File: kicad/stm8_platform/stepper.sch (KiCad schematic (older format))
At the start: 32 parts, among them J1 CONN_02X10, P1 UART, P2 SWIM, Q1 AO3401, Q2 AO3401, Q3 AO3401, SW1 SW_DIP_x03, U1 STM8S105K4T6C, U2 ULN2803A, U3 LD1117S50CTR

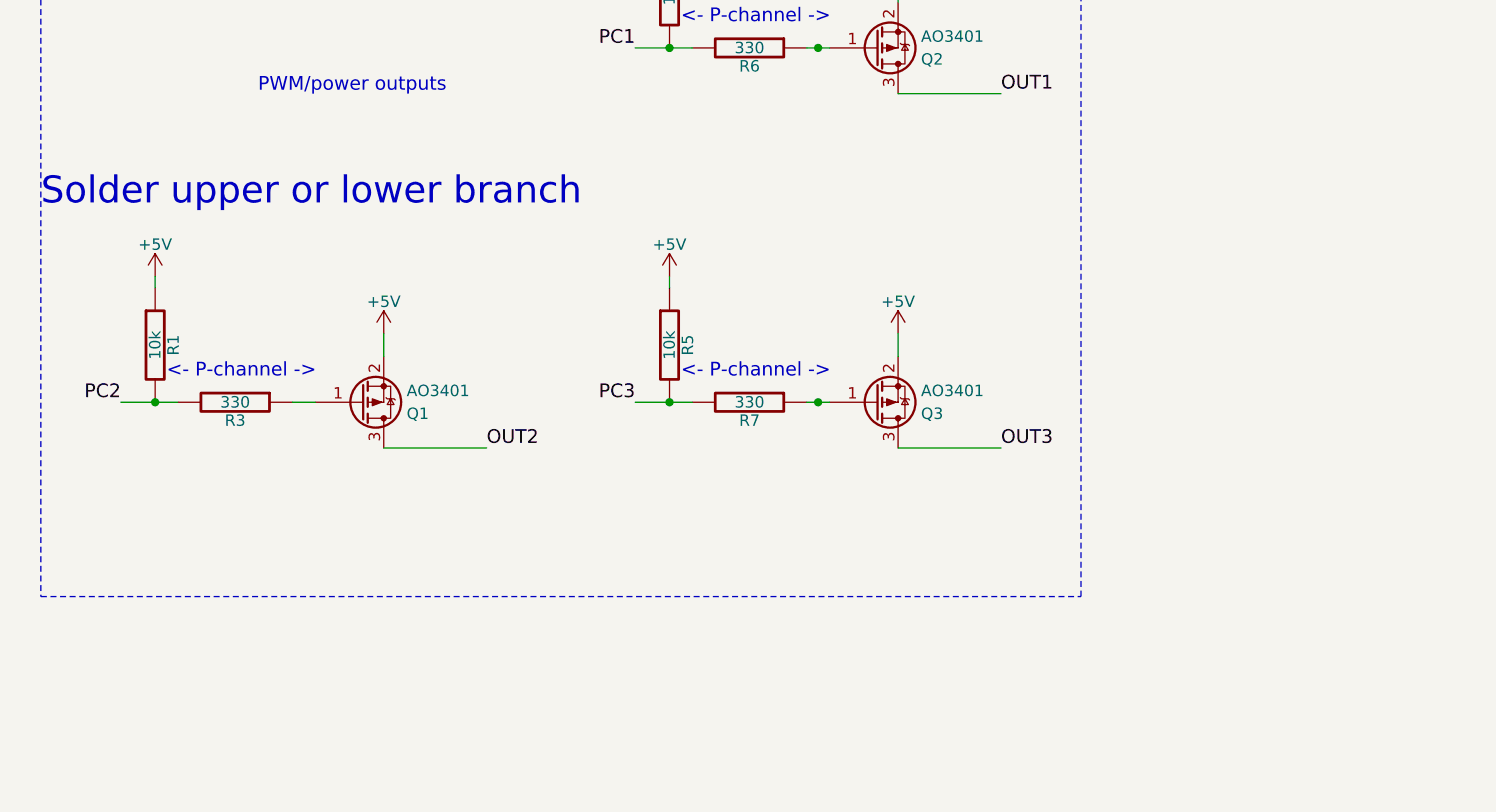
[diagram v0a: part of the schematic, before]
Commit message: small update
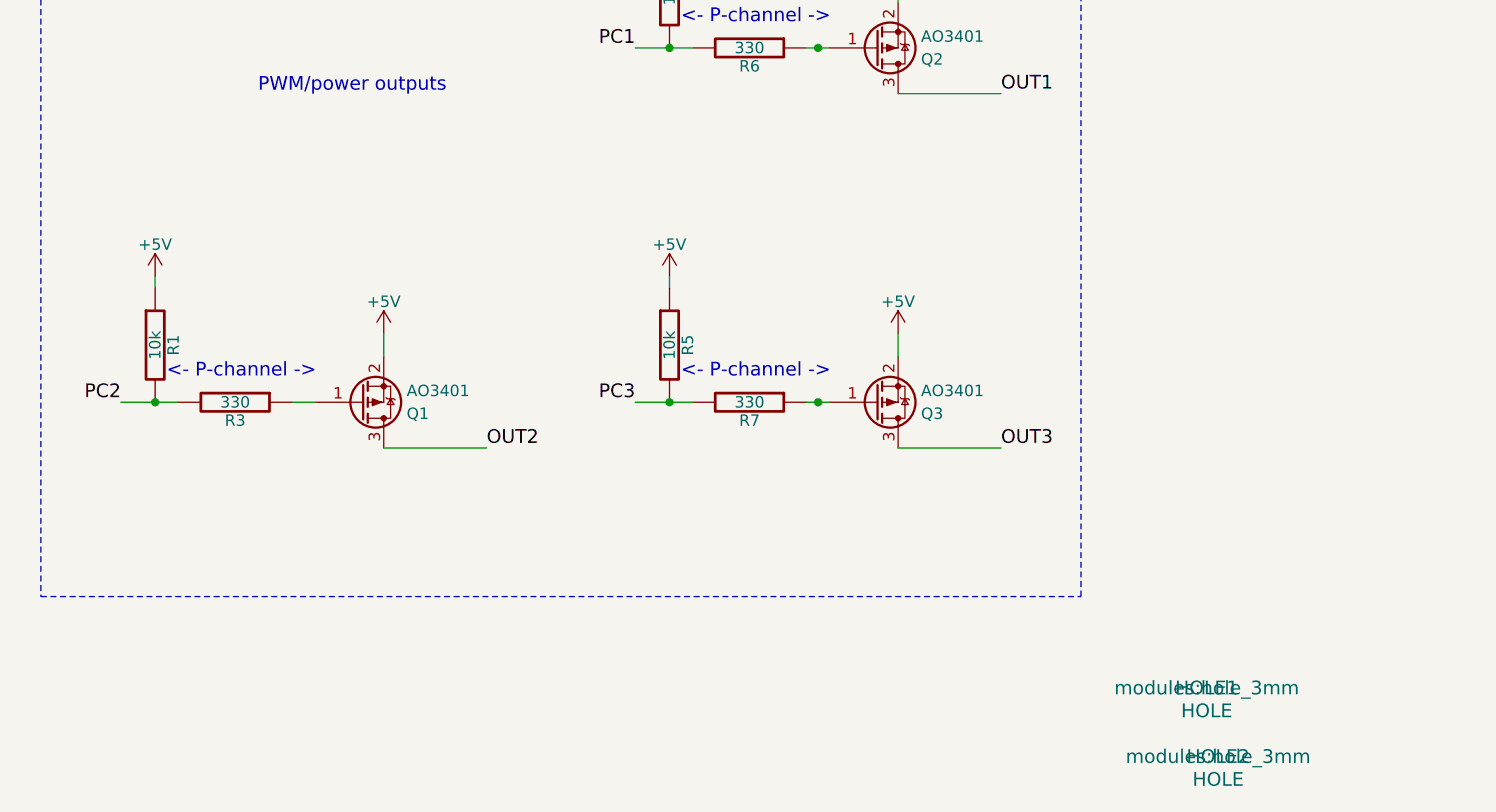
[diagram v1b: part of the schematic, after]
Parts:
- added HOLE1, HOLE2: HOLE, modules:hole_3mm, symbol HOLE
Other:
- note removed: "Solder upper or lower branch"
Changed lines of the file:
@@
 LIBS:switches
 LIBS:ESD_Protection
+LIBS:my_elements
 LIBS:stepper-cache
 EELAYER 25 0
@@
 $EndComp
 $Comp
-L GND-RESCUE-stepper #PWR01
+L GND-RESCUE-stepper #PWR5
 U 1 1 52FB03EF
 P 1500 1950
-F 0 "#PWR01" H 1500 1950 30  0001 C CNN
+F 0 "#PWR5" H 1500 1950 30  0001 C CNN
 F 1 "GND" H 1500 1880 30  0001 C CNN
 F 2 "" H 1500 1950 60  0000 C CNN
@@
 $EndComp
 $Comp
-L GND-RESCUE-stepper #PWR02
+L GND-RESCUE-stepper #PWR4
 U 1 1 52FB0400
 P 1500 1350
-F 0 "#PWR02" H 1500 1350 30  0001 C CNN
+F 0 "#PWR4" H 1500 1350 30  0001 C CNN
 F 1 "GND" H 1500 1280 30  0001 C CNN
 F 2 "" H 1500 1350 60  0000 C CNN
@@
 $EndComp
 $Comp
-L GND-RESCUE-stepper #PWR03
+L GND-RESCUE-stepper #PWR1
 U 1 1 52FB0453
 P 800 1850
-F 0 "#PWR03" H 800 1850 30  0001 C CNN
+F 0 "#PWR1" H 800 1850 30  0001 C CNN
 F 1 "GND" H 800 1780 30  0001 C CNN
 F 2 "" H 800 1850 60  0000 C CNN
@@
 $EndComp
 $Comp
-L GND-RESCUE-stepper #PWR04
+L GND-RESCUE-stepper #PWR22
 U 1 1 52FB0F03
 P 9850 1650
-F 0 "#PWR04" H 9850 1650 30  0001 C CNN
+F 0 "#PWR22" H 9850 1650 30  0001 C CNN
 F 1 "GND" H 9850 1580 30  0001 C CNN
 F 2 "" H 9850 1650 60  0000 C CNN
@@
 $EndComp
 $Comp
-L GND-RESCUE-stepper #PWR05
+L GND-RESCUE-stepper #PWR23
 U 1 1 52FB287C
 P 10150 1400
-F 0 "#PWR05" H 10150 1400 30  0001 C CNN
+F 0 "#PWR23" H 10150 1400 30  0001 C CNN
 F 1 "GND" H 10150 1330 30  0001 C CNN
 F 2 "" H 10150 1400 60  0000 C CNN
@@
 TXD
 $Comp
-L GND-RESCUE-stepper #PWR06
+L GND-RESCUE-stepper #PWR26
 U 1 1 52FB4CEF
 P 10650 2500
-F 0 "#PWR06" H 10650 2500 30  0001 C CNN
+F 0 "#PWR26" H 10650 2500 30  0001 C CNN
 F 1 "GND" H 10650 2430 30  0001 C CNN
 F 2 "" H 10650 2500 60  0000 C CNN
@@
 $EndComp
 $Comp
-L +5V #PWR07
+L +5V #PWR20
 U 1 1 5984240F
 P 9250 1050
-F 0 "#PWR07" H 9250 900 50  0001 C CNN
+F 0 "#PWR20" H 9250 900 50  0001 C CNN
 F 1 "+5V" H 9250 1190 50  0000 C CNN
 F 2 "" H 9250 1050 50  0001 C CNN
@@
 $EndComp
 $Comp
-L +5V #PWR08
+L +5V #PWR25
 U 1 1 59842472
 P 10600 1600
-F 0 "#PWR08" H 10600 1450 50  0001 C CNN
+F 0 "#PWR25" H 10600 1450 50  0001 C CNN
 F 1 "+5V" H 10600 1740 50  0000 C CNN
 F 2 "" H 10600 1600 50  0001 C CNN
@@
 $EndComp
 $Comp
-L +5V #PWR09
+L +5V #PWR2
 U 1 1 598424AD
 P 1350 1750
-F 0 "#PWR09" H 1350 1600 50  0001 C CNN
+F 0 "#PWR2" H 1350 1600 50  0001 C CNN
 F 1 "+5V" H 1350 1890 50  0000 C CNN
 F 2 "" H 1350 1750 50  0001 C CNN
@@
 $EndComp
 $Comp
-L +5V #PWR010
+L +5V #PWR7
 U 1 1 59842925
 P 2500 3650
-F 0 "#PWR010" H 2500 3500 50  0001 C CNN
+F 0 "#PWR7" H 2500 3500 50  0001 C CNN
 F 1 "+5V" H 2500 3790 50  0000 C CNN
 F 2 "" H 2500 3650 50  0001 C CNN
@@
 $EndComp
 $Comp
-L +5V #PWR011
+L +5V #PWR21
 U 1 1 59844ACD
 P 9400 3650
-F 0 "#PWR011" H 9400 3500 50  0001 C CNN
+F 0 "#PWR21" H 9400 3500 50  0001 C CNN
 F 1 "+5V" H 9400 3790 50  0000 C CNN
 F 2 "" H 9400 3650 50  0001 C CNN
@@
 $EndComp
 $Comp
-L GND-RESCUE-stepper #PWR012
+L GND-RESCUE-stepper #PWR27
 U 1 1 598456D9
 P 10700 3200
-F 0 "#PWR012" H 10700 3200 30  0001 C CNN
+F 0 "#PWR27" H 10700 3200 30  0001 C CNN
 F 1 "GND" H 10700 3130 30  0001 C CNN
 F 2 "" H 10700 3200 60  0000 C CNN
@@
 On-board LED
 $Comp
-L +5V #PWR013
+L +5V #PWR3
 U 1 1 59847EEF
 P 1350 5100
-F 0 "#PWR013" H 1350 4950 50  0001 C CNN
+F 0 "#PWR3" H 1350 4950 50  0001 C CNN
 F 1 "+5V" H 1350 5240 50  0000 C CNN
 F 2 "" H 1350 5100 50  0001 C CNN
@@
 $EndComp
 $Comp
-L +5V #PWR014
+L +5V #PWR6
 U 1 1 59848624
 P 2350 5350
-F 0 "#PWR014" H 2350 5200 50  0001 C CNN
+F 0 "#PWR6" H 2350 5200 50  0001 C CNN
 F 1 "+5V" H 2350 5490 50  0000 C CNN
 F 2 "" H 2350 5350 50  0001 C CNN
@@
 5.0V
 $Comp
-L +5V #PWR015
+L +5V #PWR24
 U 1 1 598515D1
 P 10250 2700
-F 0 "#PWR015" H 10250 2550 50  0001 C CNN
+F 0 "#PWR24" H 10250 2550 50  0001 C CNN
 F 1 "+5V" H 10250 2840 50  0000 C CNN
 F 2 "" H 10250 2700 50  0001 C CNN
@@
 $EndComp
 $Comp
-L GND-RESCUE-stepper #PWR016
+L GND-RESCUE-stepper #PWR16
 U 1 1 598534FD
 P 8200 1600
-F 0 "#PWR016" H 8200 1600 30  0001 C CNN
+F 0 "#PWR16" H 8200 1600 30  0001 C CNN
 F 1 "GND" H 8200 1530 30  0001 C CNN
 F 2 "" H 8200 1600 60  0000 C CNN
@@
 $EndComp
 $Comp
-L +5V #PWR017
+L +5V #PWR18
 U 1 1 59853D62
 P 8800 1100
-F 0 "#PWR017" H 8800 950 50  0001 C CNN
+F 0 "#PWR18" H 8800 950 50  0001 C CNN
 F 1 "+5V" H 8800 1240 50  0000 C CNN
 F 2 "" H 8800 1100 50  0001 C CNN
@@
 $EndComp
 $Comp
-L +12V #PWR018
+L +12V #PWR14
 U 1 1 59854294
 P 7650 1100
-F 0 "#PWR018" H 7650 950 50  0001 C CNN
+F 0 "#PWR14" H 7650 950 50  0001 C CNN
 F 1 "+12V" H 7650 1240 50  0000 C CNN
 F 2 "" H 7650 1100 50  0001 C CNN
@@
 ext USART
 $Comp
-L GND-RESCUE-stepper #PWR019
+L GND-RESCUE-stepper #PWR19
 U 1 1 598572C2
 P 9000 2650
-F 0 "#PWR019" H 9000 2650 30  0001 C CNN
+F 0 "#PWR19" H 9000 2650 30  0001 C CNN
 F 1 "GND" H 9000 2580 30  0001 C CNN
 F 2 "" H 9000 2650 60  0000 C CNN
@@
 $EndComp
 $Comp
-L GND-RESCUE-stepper #PWR020
+L GND-RESCUE-stepper #PWR12
 U 1 1 59857BB1
 P 6550 2200
-F 0 "#PWR020" H 6550 2200 30  0001 C CNN
+F 0 "#PWR12" H 6550 2200 30  0001 C CNN
 F 1 "GND" H 6550 2130 30  0001 C CNN
 F 2 "" H 6550 2200 60  0000 C CNN
@@
 $EndComp
 $Comp
-L +12V #PWR021
+L +12V #PWR13
 U 1 1 59858729
 P 7050 2050
-F 0 "#PWR021" H 7050 1900 50  0001 C CNN
+F 0 "#PWR13" H 7050 1900 50  0001 C CNN
 F 1 "+12V" H 7050 2190 50  0000 C CNN
 F 2 "" H 7050 2050 50  0001 C CNN
@@
 M2E2
 $Comp
-L +12V #PWR022
+L +12V #PWR17
 U 1 1 59864EE6
 P 8200 5500
-F 0 "#PWR022" H 8200 5350 50  0001 C CNN
+F 0 "#PWR17" H 8200 5350 50  0001 C CNN
 F 1 "+12V" H 8200 5640 50  0000 C CNN
 F 2 "" H 8200 5500 50  0001 C CNN
@@
 $EndComp
 $Comp
-L PWR_FLAG #FLG023
+L PWR_FLAG #FLG1
 U 1 1 598652F0
 P 8100 5500
-F 0 "#FLG023" H 8100 5575 50  0001 C CNN
+F 0 "#FLG1" H 8100 5575 50  0001 C CNN
 F 1 "PWR_FLAG" H 8100 5650 50  0001 C CNN
 F 2 "" H 8100 5500 50  0001 C CNN
@@
 $EndComp
 $Comp
-L GND-RESCUE-stepper #PWR024
+L GND-RESCUE-stepper #PWR15
 U 1 1 598655A5
 P 8050 4650
-F 0 "#PWR024" H 8050 4650 30  0001 C CNN
+F 0 "#PWR15" H 8050 4650 30  0001 C CNN
 F 1 "GND" H 8050 4580 30  0001 C CNN
 F 2 "" H 8050 4650 60  0000 C CNN
@@
 $EndComp
 $Comp
-L PWR_FLAG #FLG025
+L PWR_FLAG #FLG2
 U 1 1 5986564B
 P 8200 4600
-F 0 "#FLG025" H 8200 4675 50  0001 C CNN
+F 0 "#FLG2" H 8200 4675 50  0001 C CNN
 F 1 "PWR_FLAG" H 8200 4750 50  0001 C CNN
 F 2 "" H 8200 4600 50  0001 C CNN
@@
 $EndComp
 $Comp
-L +5V #PWR026
+L +5V #PWR9
 U 1 1 59875BF0
 P 3600 5100
-F 0 "#PWR026" H 3600 4950 50  0001 C CNN
+F 0 "#PWR9" H 3600 4950 50  0001 C CNN
 F 1 "+5V" H 3600 5240 50  0000 C CNN
 F 2 "" H 3600 5100 50  0001 C CNN
@@
 $EndComp
 $Comp
-L +5V #PWR027
+L +5V #PWR11
 U 1 1 59875BF6
 P 4600 5350
-F 0 "#PWR027" H 4600 5200 50  0001 C CNN
+F 0 "#PWR11" H 4600 5200 50  0001 C CNN
 F 1 "+5V" H 4600 5490 50  0000 C CNN
 F 2 "" H 4600 5350 50  0001 C CNN
@@
 $EndComp
 $Comp
-L +5V #PWR028
+L +5V #PWR8
 U 1 1 59876770
 P 3600 3550
-F 0 "#PWR028" H 3600 3400 50  0001 C CNN
+F 0 "#PWR8" H 3600 3400 50  0001 C CNN
 F 1 "+5V" H 3600 3690 50  0000 C CNN
 F 2 "" H 3600 3550 50  0001 C CNN
@@
 $EndComp
 $Comp
-L +5V #PWR029
+L +5V #PWR10
 U 1 1 59876776
 P 4600 3800
-F 0 "#PWR029" H 4600 3650 50  0001 C CNN
+F 0 "#PWR10" H 4600 3650 50  0001 C CNN
 F 1 "+5V" H 4600 3940 50  0000 C CNN
 F 2 "" H 4600 3800 50  0001 C CNN
@@
 Wire Notes Line
 	5400 3300 850  3300
-Text Notes 850  4800 0    118  ~ 0
-Solder upper or lower branch
 Wire Wire Line
 	8150 2850 8500 2850
@@
 	8600 2500 8250 2500
 Connection ~ 8250 2500
+$Comp
+L HOLE HOLE2
+U 1 1 59B6BC5E
+P 6000 7200
+F 0 "HOLE2" H 6000 7200 60  0000 C CNN
+F 1 "HOLE" H 6000 7100 60  0000 C CNN
+F 2 "modules:hole_3mm" H 6000 7200 60  0000 C CNN
+F 3 "" H 6000 7200 60  0000 C CNN
+	1    6000 7200
+	1    0    0    -1
+$EndComp
+$Comp
+L HOLE HOLE1
+U 1 1 59B6D60D
+P 5950 6900
+F 0 "HOLE1" H 5950 6900 60  0000 C CNN
+F 1 "HOLE" H 5950 6800 60  0000 C CNN
+F 2 "modules:hole_3mm" H 5950 6900 60  0000 C CNN
+F 3 "" H 5950 6900 60  0000 C CNN
+	1    5950 6900
+	1    0    0    -1
+$EndComp
 $EndSCHEMATC

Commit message: add code for STM8-based 2stepper management board
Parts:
- removed P2: SWIM, Pin_Headers.pretty:Pin_Header_Angled_1x04_Pitch2.54mm, symbol CONN_01X05
- added P2: SWIM, Connector_PinHeader_2.54mm.pretty:PinHeader_1x03_P2.54mm_Horizontal, symbol Conn_01x03
- SW1: symbol SW_DIP_x03 -> SW_DIP_x03-RESCUE-stepper
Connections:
- net GND: now also P2.3 (Pin_3)
- net NRST: now also P2.1 (Pin_1)
- net SWIM/PD1: now also P2.2 (Pin_2)
- no-connect marks 6 -> 5
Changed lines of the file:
@@
 $EndComp
 $Comp
-L GND-RESCUE-stepper #PWR5
+L GND-RESCUE-stepper #PWR01
 U 1 1 52FB03EF
 P 1500 1950
-F 0 "#PWR5" H 1500 1950 30  0001 C CNN
+F 0 "#PWR01" H 1500 1950 30  0001 C CNN
 F 1 "GND" H 1500 1880 30  0001 C CNN
 F 2 "" H 1500 1950 60  0000 C CNN
@@
 $EndComp
 $Comp
-L GND-RESCUE-stepper #PWR4
+L GND-RESCUE-stepper #PWR02
 U 1 1 52FB0400
 P 1500 1350
-F 0 "#PWR4" H 1500 1350 30  0001 C CNN
+F 0 "#PWR02" H 1500 1350 30  0001 C CNN
 F 1 "GND" H 1500 1280 30  0001 C CNN
 F 2 "" H 1500 1350 60  0000 C CNN
@@
 $EndComp
 $Comp
-L GND-RESCUE-stepper #PWR1
+L GND-RESCUE-stepper #PWR03
 U 1 1 52FB0453
 P 800 1850
-F 0 "#PWR1" H 800 1850 30  0001 C CNN
+F 0 "#PWR03" H 800 1850 30  0001 C CNN
 F 1 "GND" H 800 1780 30  0001 C CNN
 F 2 "" H 800 1850 60  0000 C CNN
@@
 Text Label 4550 1000 0    60   ~ 0
 PD7
-$Comp
-L CONN_01X05 P2
-U 1 1 52FB0A49
-P 10900 1350
-F 0 "P2" H 10900 1650 50  0000 C CNN
-F 1 "SWIM" H 10900 1050 50  0000 C CNN
-F 2 "Pin_Headers.pretty:Pin_Header_Angled_1x04_Pitch2.54mm" H 10900 1350 60  0001 C CNN
-F 3 "" H 10900 1350 60  0000 C CNN
-	1    10900 1350
-	1    0    0    -1
-$EndComp
 Text Label 10700 1250 2    60   ~ 0
 SWIM/PD1
@@
 $EndComp
 $Comp
-L GND-RESCUE-stepper #PWR22
+L GND-RESCUE-stepper #PWR04
 U 1 1 52FB0F03
 P 9850 1650
-F 0 "#PWR22" H 9850 1650 30  0001 C CNN
+F 0 "#PWR04" H 9850 1650 30  0001 C CNN
 F 1 "GND" H 9850 1580 30  0001 C CNN
 F 2 "" H 9850 1650 60  0000 C CNN
@@
 $EndComp
 $Comp
-L GND-RESCUE-stepper #PWR23
+L GND-RESCUE-stepper #PWR05
 U 1 1 52FB287C
 P 10150 1400
-F 0 "#PWR23" H 10150 1400 30  0001 C CNN
+F 0 "#PWR05" H 10150 1400 30  0001 C CNN
 F 1 "GND" H 10150 1330 30  0001 C CNN
 F 2 "" H 10150 1400 60  0000 C CNN
@@
 TXD
 $Comp
-L GND-RESCUE-stepper #PWR26
+L GND-RESCUE-stepper #PWR06
 U 1 1 52FB4CEF
 P 10650 2500
-F 0 "#PWR26" H 10650 2500 30  0001 C CNN
+F 0 "#PWR06" H 10650 2500 30  0001 C CNN
 F 1 "GND" H 10650 2430 30  0001 C CNN
 F 2 "" H 10650 2500 60  0000 C CNN
@@
 $EndComp
 $Comp
-L SW_DIP_x03 SW1
+L SW_DIP_x03-RESCUE-stepper SW1
 U 1 1 59834FF2
 P 9750 3950
@@
 $EndComp
 $Comp
-L +5V #PWR20
+L +5V #PWR07
 U 1 1 5984240F
 P 9250 1050
-F 0 "#PWR20" H 9250 900 50  0001 C CNN
+F 0 "#PWR07" H 9250 900 50  0001 C CNN
 F 1 "+5V" H 9250 1190 50  0000 C CNN
 F 2 "" H 9250 1050 50  0001 C CNN
@@
 $EndComp
 $Comp
-L +5V #PWR25
-U 1 1 59842472
-P 10600 1600
-F 0 "#PWR25" H 10600 1450 50  0001 C CNN
-F 1 "+5V" H 10600 1740 50  0000 C CNN
-F 2 "" H 10600 1600 50  0001 C CNN
-F 3 "" H 10600 1600 50  0001 C CNN
-	1    10600 1600
-	-1   0    0    1
-$EndComp
-$Comp
-L +5V #PWR2
+L +5V #PWR08
 U 1 1 598424AD
 P 1350 1750
-F 0 "#PWR2" H 1350 1600 50  0001 C CNN
+F 0 "#PWR08" H 1350 1600 50  0001 C CNN
 F 1 "+5V" H 1350 1890 50  0000 C CNN
 F 2 "" H 1350 1750 50  0001 C CNN
@@
 $EndComp
 $Comp
-L +5V #PWR7
+L +5V #PWR09
 U 1 1 59842925
 P 2500 3650
-F 0 "#PWR7" H 2500 3500 50  0001 C CNN
+F 0 "#PWR09" H 2500 3500 50  0001 C CNN
 F 1 "+5V" H 2500 3790 50  0000 C CNN
 F 2 "" H 2500 3650 50  0001 C CNN
@@
 $EndComp
 $Comp
-L +5V #PWR21
+L +5V #PWR010
 U 1 1 59844ACD
 P 9400 3650
-F 0 "#PWR21" H 9400 3500 50  0001 C CNN
+F 0 "#PWR010" H 9400 3500 50  0001 C CNN
 F 1 "+5V" H 9400 3790 50  0000 C CNN
 F 2 "" H 9400 3650 50  0001 C CNN
@@
 $EndComp
 $Comp
-L GND-RESCUE-stepper #PWR27
+L GND-RESCUE-stepper #PWR011
 U 1 1 598456D9
 P 10700 3200
-F 0 "#PWR27" H 10700 3200 30  0001 C CNN
+F 0 "#PWR011" H 10700 3200 30  0001 C CNN
 F 1 "GND" H 10700 3130 30  0001 C CNN
 F 2 "" H 10700 3200 60  0000 C CNN
@@
 On-board LED
 $Comp
-L +5V #PWR3
+L +5V #PWR012
 U 1 1 59847EEF
 P 1350 5100
-F 0 "#PWR3" H 1350 4950 50  0001 C CNN
+F 0 "#PWR012" H 1350 4950 50  0001 C CNN
 F 1 "+5V" H 1350 5240 50  0000 C CNN
 F 2 "" H 1350 5100 50  0001 C CNN
@@
 $EndComp
 $Comp
-L +5V #PWR6
+L +5V #PWR013
 U 1 1 59848624
 P 2350 5350
-F 0 "#PWR6" H 2350 5200 50  0001 C CNN
+F 0 "#PWR013" H 2350 5200 50  0001 C CNN
 F 1 "+5V" H 2350 5490 50  0000 C CNN
 F 2 "" H 2350 5350 50  0001 C CNN
@@
 Text Notes 1800 4300 0    60   ~ 0
 PWM/power outputs
-NoConn ~ 10700 1450
 Text Notes 10050 850  0    60   ~ 0
 SWIM
@@
 5.0V
 $Comp
-L +5V #PWR24
+L +5V #PWR014
 U 1 1 598515D1
 P 10250 2700
-F 0 "#PWR24" H 10250 2550 50  0001 C CNN
+F 0 "#PWR014" H 10250 2550 50  0001 C CNN
 F 1 "+5V" H 10250 2840 50  0000 C CNN
 F 2 "" H 10250 2700 50  0001 C CNN
@@
 $EndComp
 $Comp
-L GND-RESCUE-stepper #PWR16
+L GND-RESCUE-stepper #PWR015
 U 1 1 598534FD
 P 8200 1600
-F 0 "#PWR16" H 8200 1600 30  0001 C CNN
+F 0 "#PWR015" H 8200 1600 30  0001 C CNN
 F 1 "GND" H 8200 1530 30  0001 C CNN
 F 2 "" H 8200 1600 60  0000 C CNN
@@
 $EndComp
 $Comp
-L +5V #PWR18
+L +5V #PWR016
 U 1 1 59853D62
 P 8800 1100
-F 0 "#PWR18" H 8800 950 50  0001 C CNN
+F 0 "#PWR016" H 8800 950 50  0001 C CNN
 F 1 "+5V" H 8800 1240 50  0000 C CNN
 F 2 "" H 8800 1100 50  0001 C CNN
@@
 $EndComp
 $Comp
-L +12V #PWR14
+L +12V #PWR017
 U 1 1 59854294
 P 7650 1100
-F 0 "#PWR14" H 7650 950 50  0001 C CNN
+F 0 "#PWR017" H 7650 950 50  0001 C CNN
 F 1 "+12V" H 7650 1240 50  0000 C CNN
 F 2 "" H 7650 1100 50  0001 C CNN
@@
 ext USART
 $Comp
-L GND-RESCUE-stepper #PWR19
+L GND-RESCUE-stepper #PWR018
 U 1 1 598572C2
 P 9000 2650
-F 0 "#PWR19" H 9000 2650 30  0001 C CNN
+F 0 "#PWR018" H 9000 2650 30  0001 C CNN
 F 1 "GND" H 9000 2580 30  0001 C CNN
 F 2 "" H 9000 2650 60  0000 C CNN
@@
 $EndComp
 $Comp
-L GND-RESCUE-stepper #PWR12
+L GND-RESCUE-stepper #PWR019
 U 1 1 59857BB1
 P 6550 2200
-F 0 "#PWR12" H 6550 2200 30  0001 C CNN
+F 0 "#PWR019" H 6550 2200 30  0001 C CNN
 F 1 "GND" H 6550 2130 30  0001 C CNN
 F 2 "" H 6550 2200 60  0000 C CNN
@@
 $EndComp
 $Comp
-L +12V #PWR13
+L +12V #PWR020
 U 1 1 59858729
 P 7050 2050
-F 0 "#PWR13" H 7050 1900 50  0001 C CNN
+F 0 "#PWR020" H 7050 1900 50  0001 C CNN
 F 1 "+12V" H 7050 2190 50  0000 C CNN
 F 2 "" H 7050 2050 50  0001 C CNN
@@
 M2E2
 $Comp
-L +12V #PWR17
+L +12V #PWR021
 U 1 1 59864EE6
 P 8200 5500
-F 0 "#PWR17" H 8200 5350 50  0001 C CNN
+F 0 "#PWR021" H 8200 5350 50  0001 C CNN
 F 1 "+12V" H 8200 5640 50  0000 C CNN
 F 2 "" H 8200 5500 50  0001 C CNN
@@
 $EndComp
 $Comp
-L PWR_FLAG #FLG1
+L PWR_FLAG #FLG022
 U 1 1 598652F0
 P 8100 5500
-F 0 "#FLG1" H 8100 5575 50  0001 C CNN
+F 0 "#FLG022" H 8100 5575 50  0001 C CNN
 F 1 "PWR_FLAG" H 8100 5650 50  0001 C CNN
 F 2 "" H 8100 5500 50  0001 C CNN
@@
 $EndComp
 $Comp
-L GND-RESCUE-stepper #PWR15
+L GND-RESCUE-stepper #PWR023
 U 1 1 598655A5
 P 8050 4650
-F 0 "#PWR15" H 8050 4650 30  0001 C CNN
+F 0 "#PWR023" H 8050 4650 30  0001 C CNN
 F 1 "GND" H 8050 4580 30  0001 C CNN
 F 2 "" H 8050 4650 60  0000 C CNN
@@
 $EndComp
 $Comp
-L PWR_FLAG #FLG2
+L PWR_FLAG #FLG024
 U 1 1 5986564B
 P 8200 4600
-F 0 "#FLG2" H 8200 4675 50  0001 C CNN
+F 0 "#FLG024" H 8200 4675 50  0001 C CNN
 F 1 "PWR_FLAG" H 8200 4750 50  0001 C CNN
 F 2 "" H 8200 4600 50  0001 C CNN
@@
 Wire Wire Line
 	10150 1350 10700 1350
-Wire Wire Line
-	10700 1550 10600 1550
-Wire Wire Line
-	10600 1550 10600 1600
 Wire Wire Line
 	9250 1050 9250 1150
@@
 $EndComp
 $Comp
-L +5V #PWR9
+L +5V #PWR025
 U 1 1 59875BF0
 P 3600 5100
-F 0 "#PWR9" H 3600 4950 50  0001 C CNN
+F 0 "#PWR025" H 3600 4950 50  0001 C CNN
 F 1 "+5V" H 3600 5240 50  0000 C CNN
 F 2 "" H 3600 5100 50  0001 C CNN
@@
 $EndComp
 $Comp
-L +5V #PWR11
+L +5V #PWR026
 U 1 1 59875BF6
 P 4600 5350
-F 0 "#PWR11" H 4600 5200 50  0001 C CNN
+F 0 "#PWR026" H 4600 5200 50  0001 C CNN
 F 1 "+5V" H 4600 5490 50  0000 C CNN
 F 2 "" H 4600 5350 50  0001 C CNN
@@
 $EndComp
 $Comp
-L +5V #PWR8
+L +5V #PWR027
 U 1 1 59876770
 P 3600 3550
-F 0 "#PWR8" H 3600 3400 50  0001 C CNN
+F 0 "#PWR027" H 3600 3400 50  0001 C CNN
 F 1 "+5V" H 3600 3690 50  0000 C CNN
 F 2 "" H 3600 3550 50  0001 C CNN
@@
 $EndComp
 $Comp
-L +5V #PWR10
+L +5V #PWR028
 U 1 1 59876776
 P 4600 3800
-F 0 "#PWR10" H 4600 3650 50  0001 C CNN
+F 0 "#PWR028" H 4600 3650 50  0001 C CNN
 F 1 "+5V" H 4600 3940 50  0000 C CNN
 F 2 "" H 4600 3800 50  0001 C CNN
@@
 	1    0    0    -1
 $EndComp
+$Comp
+L Conn_01x03 P2
+U 1 1 5BB234EF
+P 10900 1250
+F 0 "P2" H 10900 1450 50  0000 C CNN
+F 1 "SWIM" H 10900 1050 50  0000 C CNN
+F 2 "Connector_PinHeader_2.54mm.pretty:PinHeader_1x03_P2.54mm_Horizontal" H 10900 1250 50  0001 C CNN
+F 3 "" H 10900 1250 50  0001 C CNN
+	1    10900 1250
+	1    0    0    -1
+$EndComp
